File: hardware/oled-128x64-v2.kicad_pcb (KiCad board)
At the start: 2 copper layers, 40 x 40 mm, 34 parts, among them P1 CON-SENSOR2, P2 DEBUG, P3 BOOT, U1 XMC130024, U3 OLED013, U4 DRILL, U5 DRILL, U6 DRILL, U7 DRILL

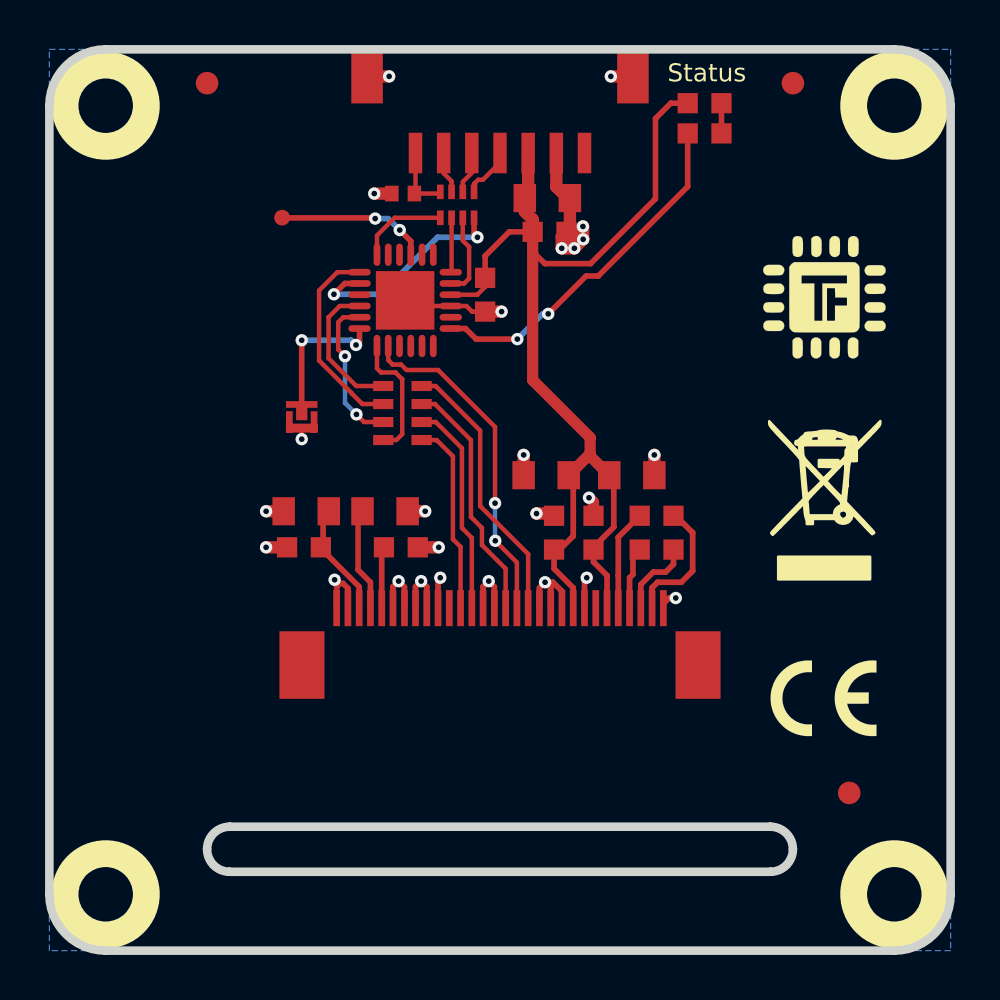
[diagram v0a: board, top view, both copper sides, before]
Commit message: move to new kicad version
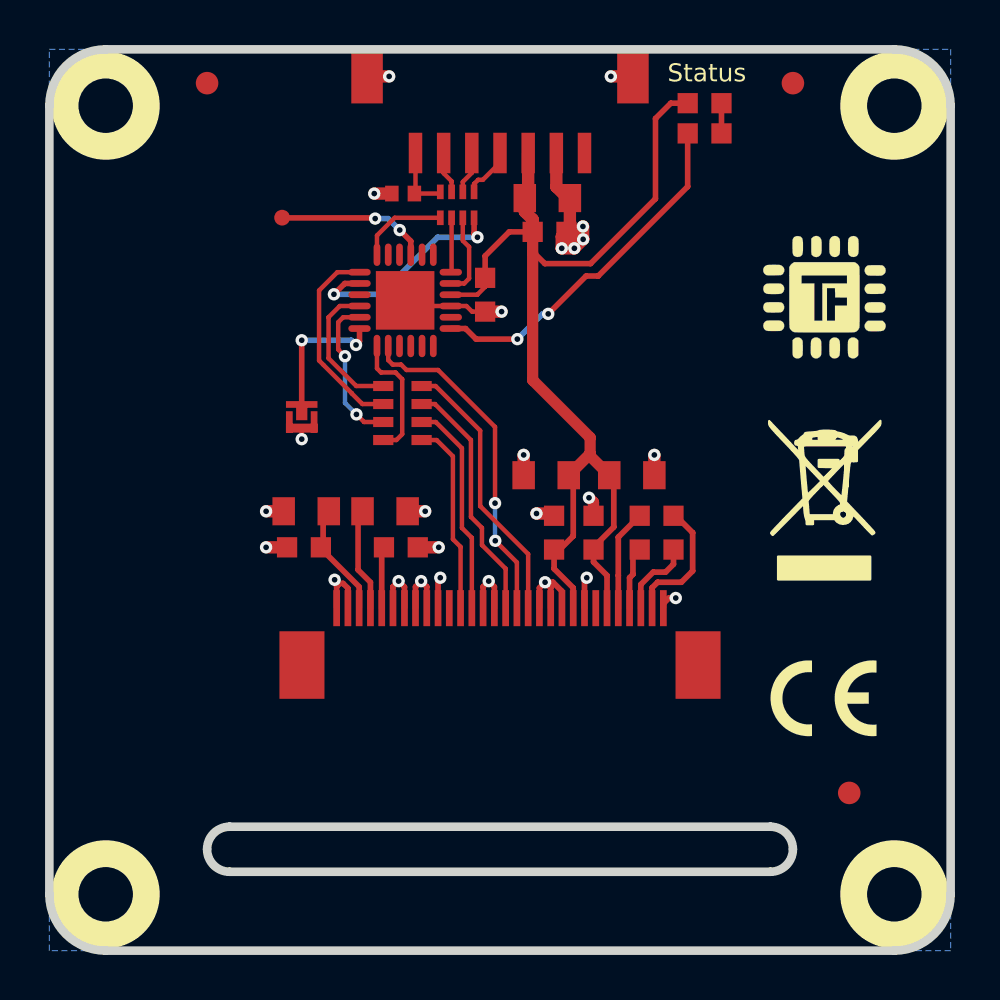
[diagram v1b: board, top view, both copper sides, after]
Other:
- net class Default removed
